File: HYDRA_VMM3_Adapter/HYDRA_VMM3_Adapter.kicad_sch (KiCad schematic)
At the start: 6 parts, among them J1 ME1014010101011, J2 ME1014010101011, J3 ME1014010101011, J4 ME1014010101011, J5 ME1014010101011, J6 ME1014010101011

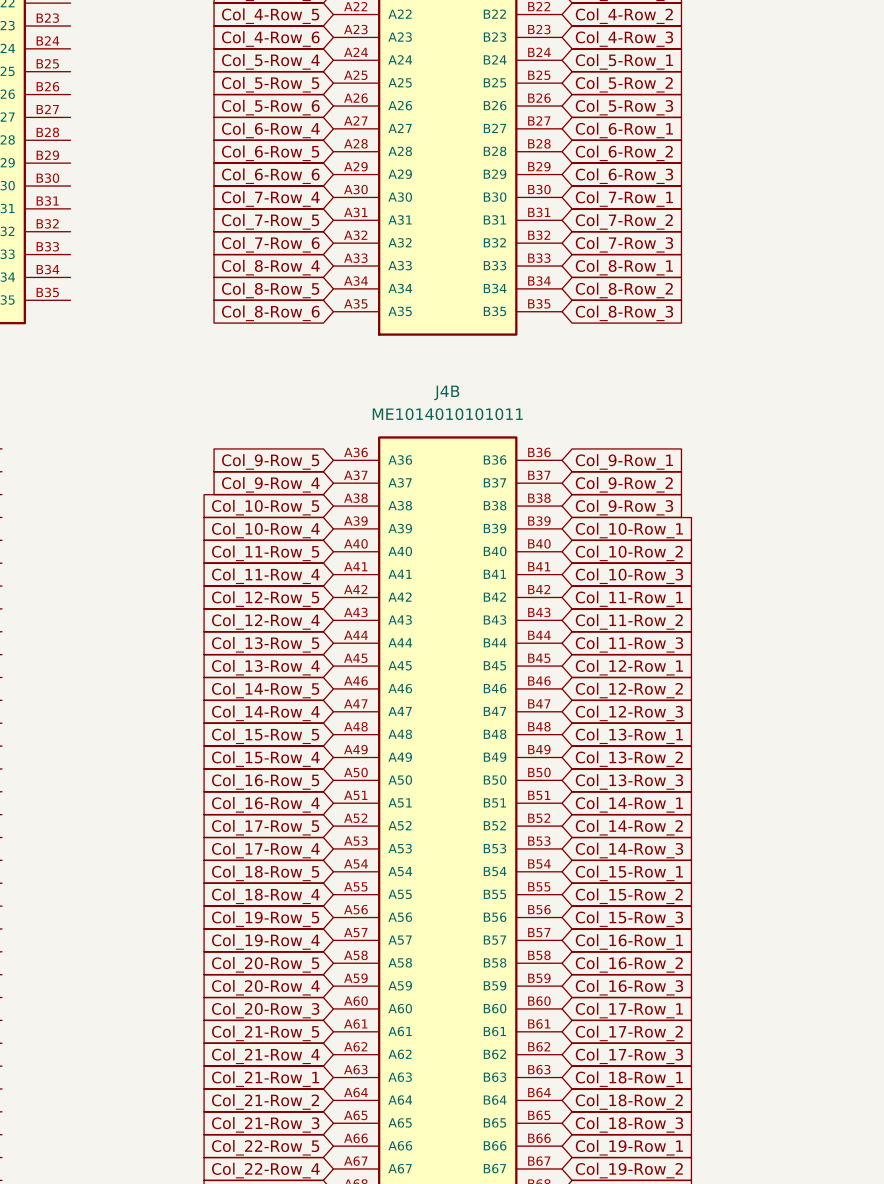
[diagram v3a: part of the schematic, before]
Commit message: .
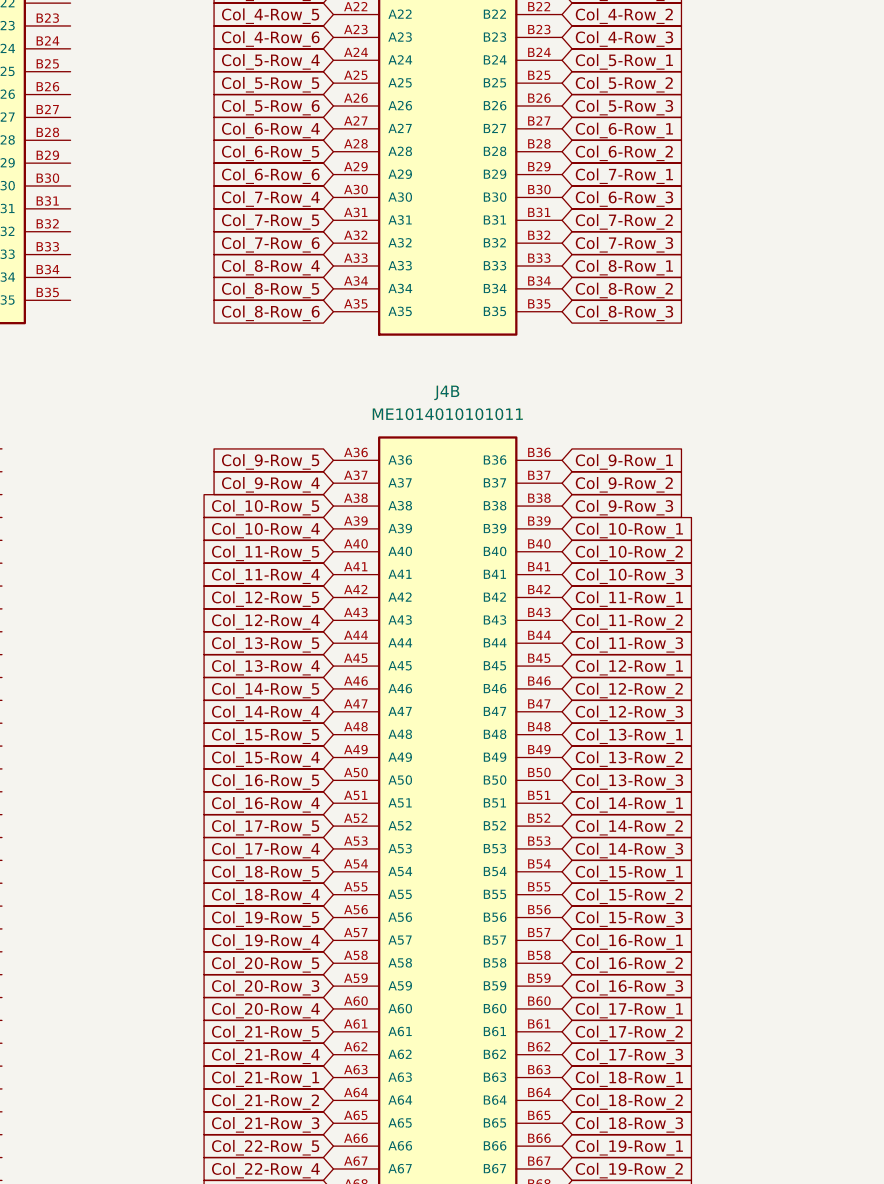
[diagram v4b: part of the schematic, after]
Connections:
- net Col_20-Row_3: now also J4.A59; no longer J4.A60
- net Col_20-Row_4: now also J4.A60; no longer J4.A59
- net Col_6-Row_3: now also J4.B30; no longer J4.B29
- net Col_7-Row_1: now also J4.B29; no longer J4.B30

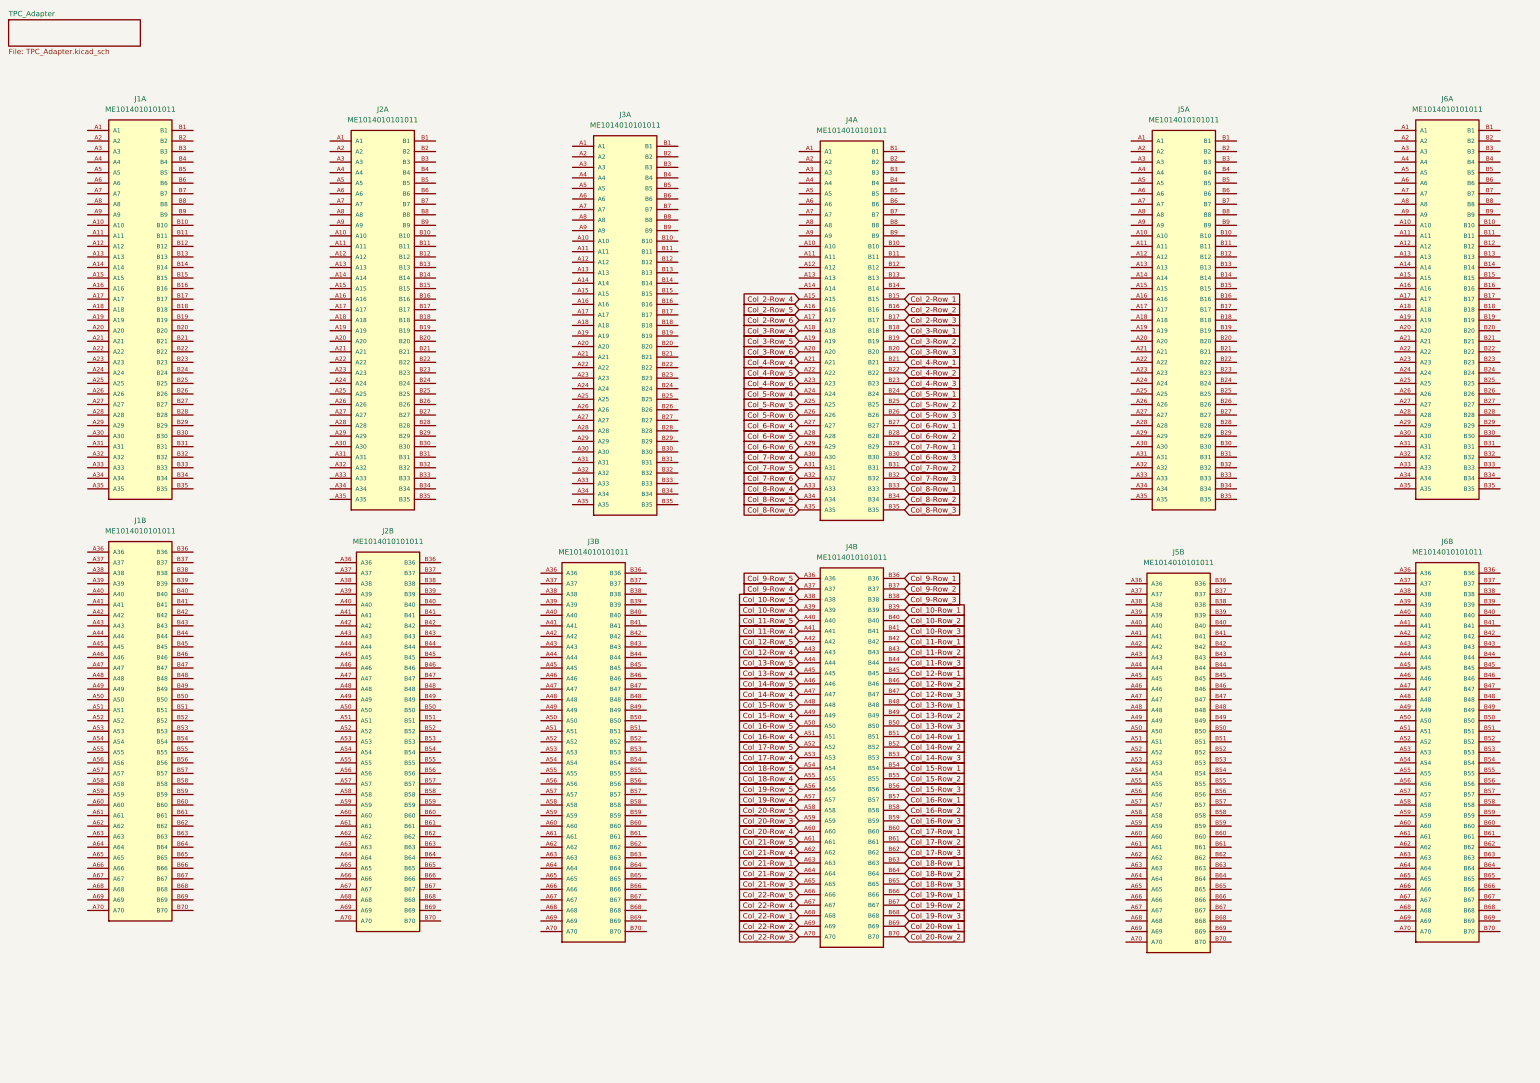
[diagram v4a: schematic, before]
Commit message: .
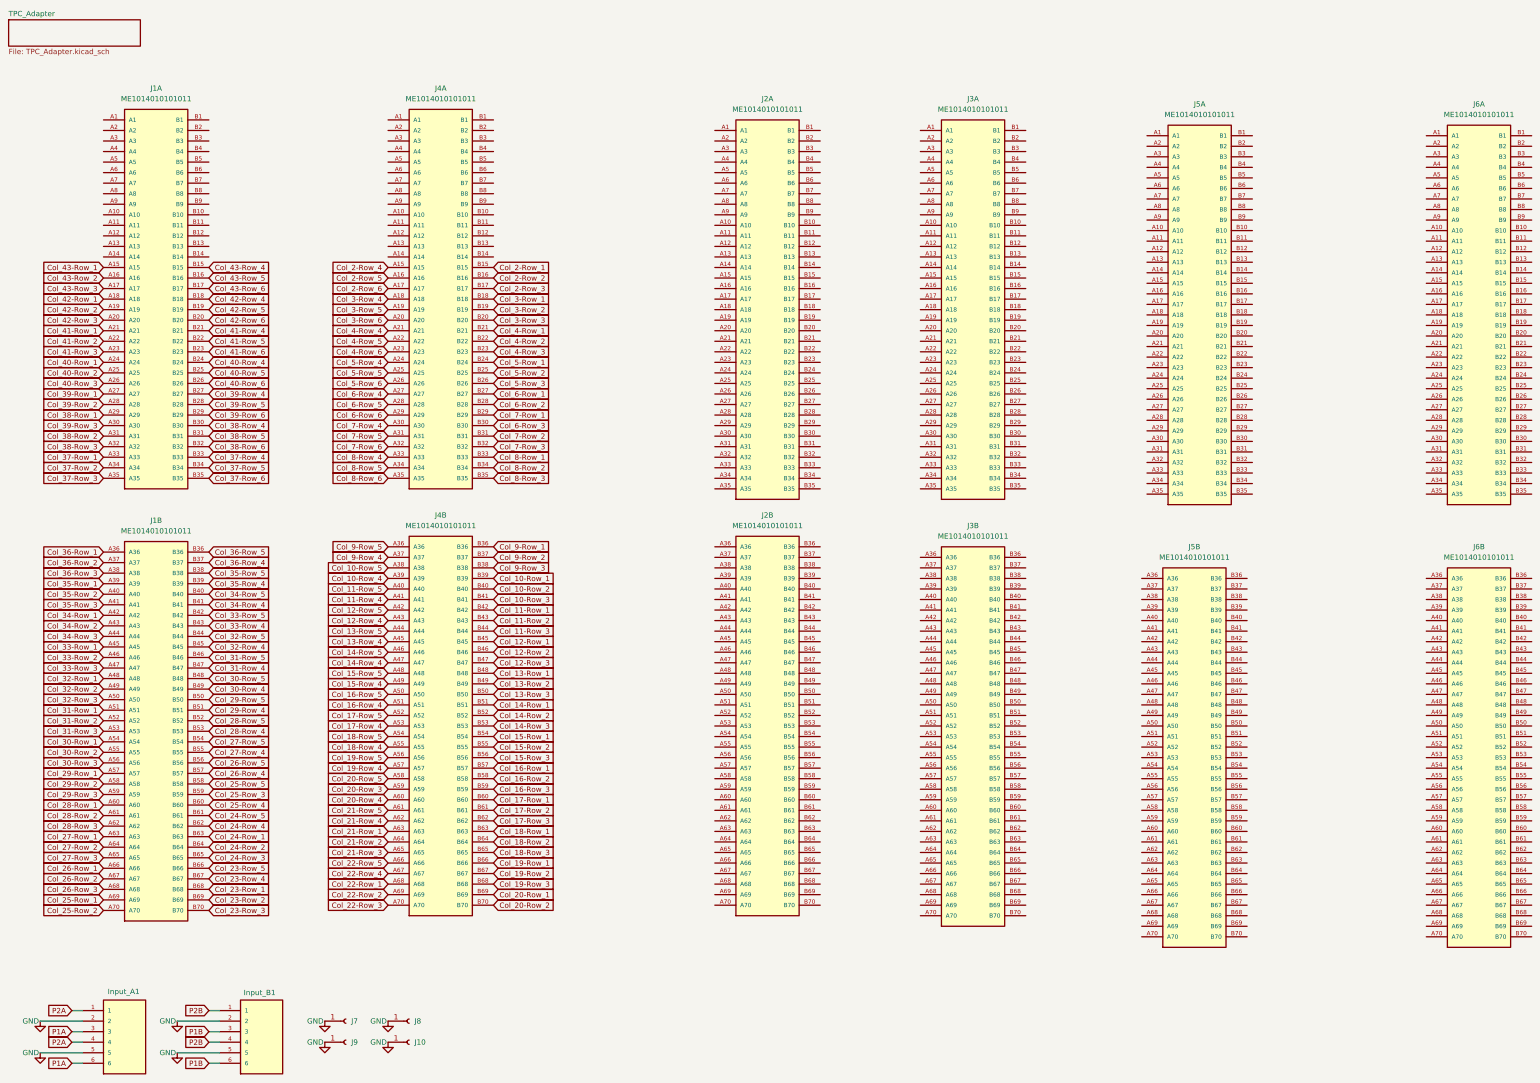
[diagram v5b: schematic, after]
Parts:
- added Input_A1, Input_B1: 39-30-1060, Molex_PCB_Power_Connector:MOLEX_39-30-1060, symbol Molex_PCB_Power_Connector:39-30-1060
- added J10, J7, J8, J9: Conn_01x01_Socket, MountingHole:MountingHole_3.2mm_M3_DIN965_Pad, symbol Connector:Conn_01x01_Socket
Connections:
- net Col_43-Row_1: now reaches J1.A15
- net Col_43-Row_2: now reaches J1.A16
- net Col_43-Row_3: now reaches J1.A17
- net Col_42-Row_1: now reaches J1.A18
- net Col_42-Row_2: now reaches J1.A19
- net Col_42-Row_3: now reaches J1.A20
- net Col_41-Row_1: now reaches J1.A21
- net Col_41-Row_2: now reaches J1.A22
- net Col_41-Row_3: now reaches J1.A23
- net Col_40-Row_1: now reaches J1.A24
- net Col_40-Row_2: now reaches J1.A25
- net Col_40-Row_3: now reaches J1.A26
- net Col_39-Row_1: now reaches J1.A27
- net Col_39-Row_2: now reaches J1.A28
- net Col_38-Row_1: now reaches J1.A29
- net Col_39-Row_3: now reaches J1.A30
- net Col_38-Row_2: now reaches J1.A31
- net Col_38-Row_3: now reaches J1.A32
- net Col_37-Row_1: now reaches J1.A33
- net Col_37-Row_2: now reaches J1.A34
- net Col_37-Row_3: now reaches J1.A35
- net Col_43-Row_4: now reaches J1.B15
- net Col_43-Row_5: now reaches J1.B16
- net Col_43-Row_6: now reaches J1.B17
- net Col_42-Row_4: now reaches J1.B18
- net Col_42-Row_5: now reaches J1.B19
- net Col_42-Row_6: now reaches J1.B20
- net Col_41-Row_4: now reaches J1.B21
- net Col_41-Row_5: now reaches J1.B22
- net Col_41-Row_6: now reaches J1.B23
- net Col_40-Row_4: now reaches J1.B24
- net Col_40-Row_5: now reaches J1.B25
- net Col_40-Row_6: now reaches J1.B26
- net Col_39-Row_4: now reaches J1.B27
- net Col_39-Row_5: now reaches J1.B28
- net Col_39-Row_6: now reaches J1.B29
- net Col_38-Row_4: now reaches J1.B30
- net Col_38-Row_5: now reaches J1.B31
- net Col_38-Row_6: now reaches J1.B32
- net Col_37-Row_4: now reaches J1.B33
- net Col_37-Row_5: now reaches J1.B34
- net Col_37-Row_6: now reaches J1.B35
- net Col_36-Row_1: now reaches J1.A36
- net Col_36-Row_2: now reaches J1.A37
- net Col_36-Row_3: now reaches J1.A38
- net Col_35-Row_1: now reaches J1.A39
- net Col_35-Row_2: now reaches J1.A40
- net Col_35-Row_3: now reaches J1.A41
- net Col_34-Row_1: now reaches J1.A42
- net Col_34-Row_2: now reaches J1.A43
- net Col_34-Row_3: now reaches J1.A44
- net Col_33-Row_1: now reaches J1.A45
- net Col_33-Row_2: now reaches J1.A46
- net Col_33-Row_3: now reaches J1.A47
- net Col_32-Row_1: now reaches J1.A48
- net Col_32-Row_2: now reaches J1.A49
- net Col_32-Row_3: now reaches J1.A50
- net Col_31-Row_1: now reaches J1.A51
- net Col_31-Row_2: now reaches J1.A52
- net Col_31-Row_3: now reaches J1.A53
- net Col_30-Row_1: now reaches J1.A54
- net Col_30-Row_2: now reaches J1.A55
- net Col_30-Row_3: now reaches J1.A56
- net Col_29-Row_1: now reaches J1.A57
- net Col_29-Row_2: now reaches J1.A58
- net Col_29-Row_3: now reaches J1.A59
- net Col_28-Row_1: now reaches J1.A60
- net Col_28-Row_2: now reaches J1.A61
- net Col_28-Row_3: now reaches J1.A62
- net Col_27-Row_1: now reaches J1.A63
- net Col_27-Row_2: now reaches J1.A64
- net Col_27-Row_3: now reaches J1.A65
- net Col_26-Row_1: now reaches J1.A66
- net Col_26-Row_2: now reaches J1.A67
- net Col_26-Row_3: now reaches J1.A68
- net Col_25-Row_1: now reaches J1.A69
- net Col_25-Row_2: now reaches J1.A70
- net Col_36-Row_5: now reaches J1.B36
- net Col_36-Row_4: now reaches J1.B37
- net Col_35-Row_5: now reaches J1.B38
- net Col_35-Row_4: now reaches J1.B39
- net Col_34-Row_5: now reaches J1.B40
- net Col_34-Row_4: now reaches J1.B41
- net Col_33-Row_5: now reaches J1.B42
- net Col_33-Row_4: now reaches J1.B43
- net Col_32-Row_5: now reaches J1.B44
- net Col_32-Row_4: now reaches J1.B45
- net Col_31-Row_5: now reaches J1.B46
- net Col_31-Row_4: now reaches J1.B47
- net Col_30-Row_5: now reaches J1.B48
- net Col_30-Row_4: now reaches J1.B49
- net Col_29-Row_5: now reaches J1.B50
- net Col_29-Row_4: now reaches J1.B51
- net Col_28-Row_5: now reaches J1.B52
- net Col_28-Row_4: now reaches J1.B53
- net Col_27-Row_5: now reaches J1.B54
- net Col_27-Row_4: now reaches J1.B55
- net Col_26-Row_5: now reaches J1.B56
- net Col_26-Row_4: now reaches J1.B57
- net Col_25-Row_5: now reaches J1.B58
- net Col_25-Row_3: now reaches J1.B59
- net Col_25-Row_4: now reaches J1.B60
- net Col_24-Row_5: now reaches J1.B61
- net Col_24-Row_4: now reaches J1.B62
- net Col_24-Row_1: now reaches J1.B63
- net Col_24-Row_2: now reaches J1.B64
- net Col_24-Row_3: now reaches J1.B65
- net Col_23-Row_5: now reaches J1.B66
- net Col_23-Row_4: now reaches J1.B67
- net Col_23-Row_1: now reaches J1.B68
- net Col_23-Row_2: now reaches J1.B69
- net Col_23-Row_3: now reaches J1.B70
- new net GND: Input_A1.2, Input_A1.5, Input_B1.2, Input_B1.5, J10.1 (Pin_1), J7.1 (Pin_1), J8.1 (Pin_1), J9.1 (Pin_1)
- new net P1A: Input_A1.3, Input_A1.6
- new net P1B: Input_B1.3, Input_B1.6
- new net P2A: Input_A1.1, Input_A1.4
- new net P2B: Input_B1.1, Input_B1.4
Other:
- moved on the sheet: J1A, J1B, J2A, J2B, J3A, J3B, J4A, J4B, J5A, J5B, J6A, J6B
